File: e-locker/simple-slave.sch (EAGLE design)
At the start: 41 parts, among them IC1 REG1117, Q1 16MHz, U1 ATMEGA328, U2 MAX487ESA+TCBX, X1 JST-XH-02-PIN-LONG-PAD, X10 JST-XH-04-PIN-LONG-PAD, X2 JST-XH-05-PIN-LONG-PAD, X3 JST-XH-04-PIN-LONG-PAD, X4 JST-XH-04-PIN-LONG-PAD, X5 JST-XH-04-PIN-LONG-PAD, X6 JST-XH-04-PIN-LONG-PAD, X7 JST-XH-04-PIN-LONG-PAD, X8 JST-XH-04-PIN-LONG-PAD, X9 JST-XH-04-PIN-LONG-PAD

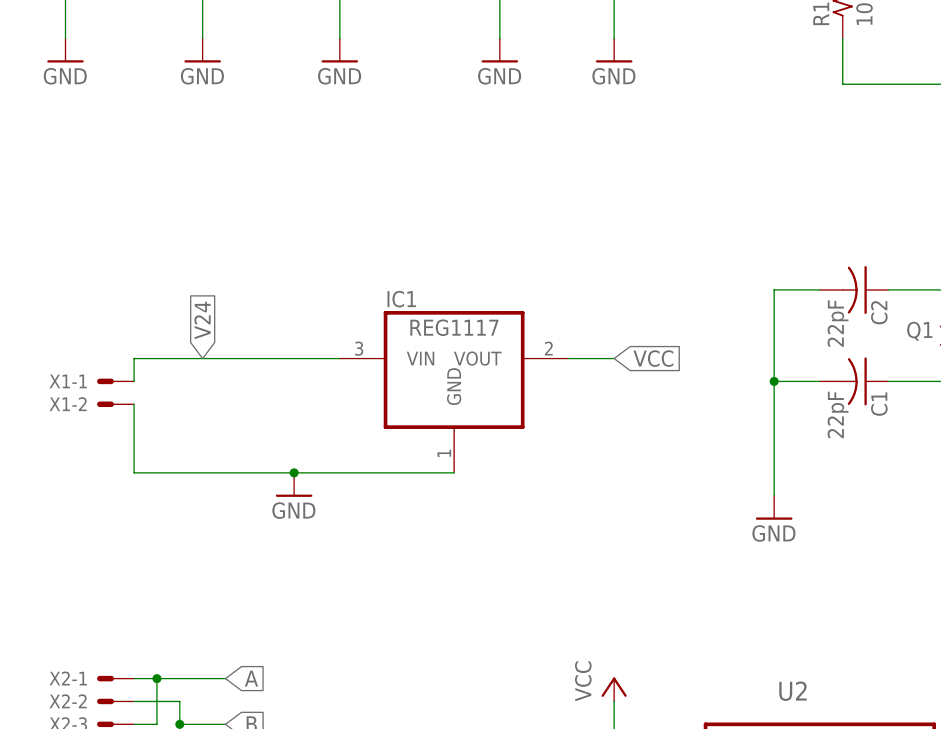
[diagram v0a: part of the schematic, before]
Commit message: changes
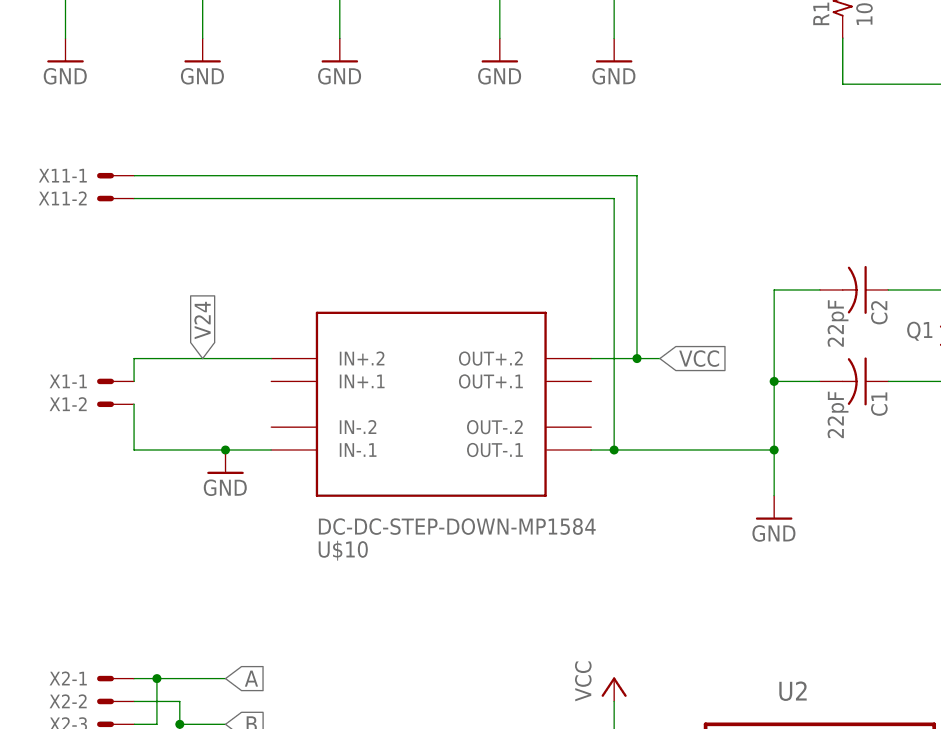
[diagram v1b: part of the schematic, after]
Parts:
- removed IC1: REG1117, burr-brown:REG1117
- added U$10: DC-DC-STEP-DOWN-MP1584, diy-modules:DC-DC-STEP-DOWN-MP1584
- added X11: JST-XH-02-PIN-LONG-PAD, Rembrandt Electronics - JST XH Connectors v1-0:JST-XH-02-PIN-LONG-PAD
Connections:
- net GND: now also U$10.IN-.1, U$10.OUT-.1, X11-2.S; no longer IC1.GND
- net V24: now also U$10.IN+.2; no longer IC1.VIN
- net VCC: now also U$10.OUT+.2, X11-1.S; no longer IC1.VOUT
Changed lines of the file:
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@@
 <?xml version="1.0" encoding="utf-8"?>
 <!DOCTYPE eagle SYSTEM "eagle.dtd">
-<eagle version="9.6.2">
+<eagle version="9.2.2">
 <drawing>
 <settings>
@@
 <part name="GND5" library="SparkFun" deviceset="GND" device=""/>
 <part name="P+7" library="SparkFun" deviceset="VCC" device=""/>
-<part name="IC1" library="burr-brown" library_urn="urn:adsk.eagle:library:111" deviceset="REG1117" device="" package3d_urn="urn:adsk.eagle:package:4940/1"/>
 <part name="U$1" library="dawidkulpa_dev" deviceset="MOSFET-N" device="TO252"/>
 <part name="U$2" library="dawidkulpa_dev" deviceset="MOSFET-N" device="TO252"/>
@@
 <part name="C7" library="rcl" library_urn="urn:adsk.eagle:library:334" deviceset="CPOL-EU" device="SANYO_SMD_C6" package3d_urn="urn:adsk.eagle:package:23465/1"/>
 <part name="C8" library="adafruit" deviceset="C-US" device="C0805" value="0.1uF"/>
+<part name="U$10" library="diy-modules" deviceset="DC-DC-STEP-DOWN-MP1584" device=""/>
+<part name="X11" library="Rembrandt Electronics - JST XH Connectors v1-0" deviceset="JST-XH-02-PIN" device="-LONG-PAD"/>
 </parts>
 <sheets>
@@
 <instance part="P+7" gate="1" x="114.3" y="210.82" smashed="yes">
 <attribute name="VALUE" x="113.284" y="214.376" size="1.778" layer="96"/>
-</instance>
-<instance part="IC1" gate="G$1" x="96.52" y="157.48" smashed="yes">
-<attribute name="NAME" x="88.9" y="163.195" size="1.778" layer="95" ratio="10"/>
-<attribute name="VALUE" x="91.44" y="160.02" size="1.778" layer="96" ratio="10"/>
 </instance>
 <instance part="U$1" gate="G$1" x="350.52" y="203.2" smashed="yes" rot="R90"/>
@@
 <attribute name="VALUE" x="287.02" y="106.045" size="1.778" layer="96"/>
 </instance>
-<instance part="GND9" gate="1" x="78.74" y="142.24" smashed="yes">
-<attribute name="VALUE" x="76.2" y="139.7" size="1.778" layer="96"/>
+<instance part="GND9" gate="1" x="71.12" y="144.78" smashed="yes">
+<attribute name="VALUE" x="68.58" y="142.24" size="1.778" layer="96"/>
 </instance>
 <instance part="GND10" gate="1" x="66.04" y="91.44" smashed="yes">
@@
 <attribute name="NAME" x="69.596" y="203.835" size="1.778" layer="95"/>
 <attribute name="VALUE" x="69.596" y="199.009" size="1.778" layer="96"/>
+</instance>
+<instance part="U$10" gate="G$1" x="93.98" y="152.4" smashed="yes" rot="MR180">
+<attribute name="NAME" x="81.28" y="137.16" size="1.778" layer="95" rot="MR180"/>
+<attribute name="VALUE" x="81.28" y="139.7" size="1.778" layer="96" rot="MR180"/>
+</instance>
+<instance part="X11" gate="-2" x="58.42" y="175.26" smashed="yes" rot="R180">
+<attribute name="NAME" x="55.88" y="176.022" size="1.524" layer="95" rot="R180"/>
+</instance>
+<instance part="X11" gate="-1" x="58.42" y="177.8" smashed="yes" rot="R180">
+<attribute name="NAME" x="55.88" y="178.562" size="1.524" layer="95" rot="R180"/>
 </instance>
 </instances>
@@
 <wire x1="132.08" y1="165.1" x2="132.08" y2="154.94" width="0.1524" layer="91"/>
 <pinref part="C1" gate="G$1" pin="2"/>
-<wire x1="132.08" y1="154.94" x2="132.08" y2="142.24" width="0.1524" layer="91"/>
+<wire x1="132.08" y1="154.94" x2="132.08" y2="147.32" width="0.1524" layer="91"/>
+<wire x1="132.08" y1="147.32" x2="132.08" y2="142.24" width="0.1524" layer="91"/>
 <wire x1="137.16" y1="154.94" x2="132.08" y2="154.94" width="0.1524" layer="91"/>
 <junction x="132.08" y="154.94"/>
 <pinref part="GND1" gate="1" pin="GND"/>
+<pinref part="U$10" gate="G$1" pin="OUT-.1"/>
+<wire x1="111.76" y1="147.32" x2="114.3" y2="147.32" width="0.1524" layer="91"/>
+<junction x="132.08" y="147.32"/>
+<pinref part="X11" gate="-2" pin="S"/>
+<wire x1="114.3" y1="147.32" x2="132.08" y2="147.32" width="0.1524" layer="91"/>
+<wire x1="60.96" y1="175.26" x2="114.3" y2="175.26" width="0.1524" layer="91"/>
+<wire x1="114.3" y1="175.26" x2="114.3" y2="147.32" width="0.1524" layer="91"/>
+<junction x="114.3" y="147.32"/>
 </segment>
 <segment>
@@
 </segment>
 <segment>
-<pinref part="IC1" gate="G$1" pin="GND"/>
-<wire x1="96.52" y1="144.78" x2="78.74" y2="144.78" width="0.1524" layer="91"/>
 <pinref part="X1" gate="-2" pin="S"/>
-<wire x1="78.74" y1="144.78" x2="60.96" y2="144.78" width="0.1524" layer="91"/>
-<wire x1="60.96" y1="152.4" x2="60.96" y2="144.78" width="0.1524" layer="91"/>
+<wire x1="71.12" y1="147.32" x2="60.96" y2="147.32" width="0.1524" layer="91"/>
+<wire x1="60.96" y1="152.4" x2="60.96" y2="147.32" width="0.1524" layer="91"/>
 <pinref part="GND9" gate="1" pin="GND"/>
-<junction x="78.74" y="144.78"/>
+<pinref part="U$10" gate="G$1" pin="IN-.1"/>
+<wire x1="71.12" y1="147.32" x2="76.2" y2="147.32" width="0.1524" layer="91"/>
+<junction x="71.12" y="147.32"/>
 </segment>
 <segment>
@@
 </segment>
 <segment>
-<pinref part="IC1" gate="G$1" pin="VOUT"/>
-<wire x1="109.22" y1="157.48" x2="114.3" y2="157.48" width="0.1524" layer="91"/>
-<label x="114.3" y="157.48" size="1.778" layer="95" xref="yes"/>
+<pinref part="U$10" gate="G$1" pin="OUT+.2"/>
+<wire x1="111.76" y1="157.48" x2="116.84" y2="157.48" width="0.1524" layer="91"/>
+<label x="119.38" y="157.48" size="1.778" layer="95" xref="yes"/>
+<pinref part="X11" gate="-1" pin="S"/>
+<wire x1="116.84" y1="157.48" x2="119.38" y2="157.48" width="0.1524" layer="91"/>
+<wire x1="60.96" y1="177.8" x2="116.84" y2="177.8" width="0.1524" layer="91"/>
+<wire x1="116.84" y1="177.8" x2="116.84" y2="157.48" width="0.1524" layer="91"/>
+<junction x="116.84" y="157.48"/>
 </segment>
 </net>
@@
 <net name="V24" class="0">
 <segment>
-<pinref part="IC1" gate="G$1" pin="VIN"/>
-<wire x1="83.82" y1="157.48" x2="60.96" y2="157.48" width="0.1524" layer="91"/>
 <pinref part="X1" gate="-1" pin="S"/>
 <wire x1="60.96" y1="154.94" x2="60.96" y2="157.48" width="0.1524" layer="91"/>
 <label x="68.58" y="157.48" size="1.778" layer="95" rot="R90" xref="yes"/>
-</segment>
-<segment>
+<pinref part="U$10" gate="G$1" pin="IN+.2"/>
+<wire x1="60.96" y1="157.48" x2="76.2" y2="157.48" width="0.1524" layer="91"/>
+</segment>
+<segment>
